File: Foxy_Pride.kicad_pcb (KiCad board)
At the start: 2 copper layers, 89.3 x 67.9 mm, 34 parts, among them U1 TLC555CDR, U2 74HC4017D

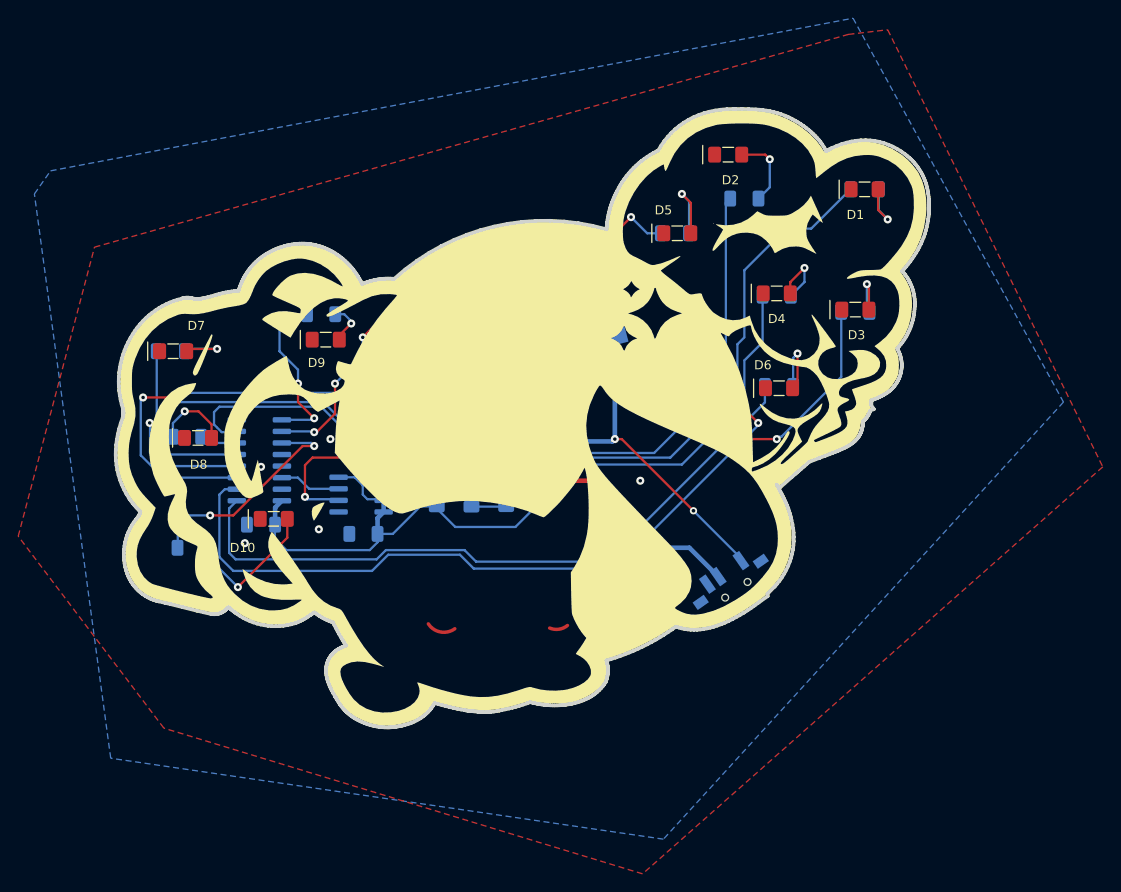
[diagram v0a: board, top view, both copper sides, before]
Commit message: Finalized design and layout on Foxy Pride PCB
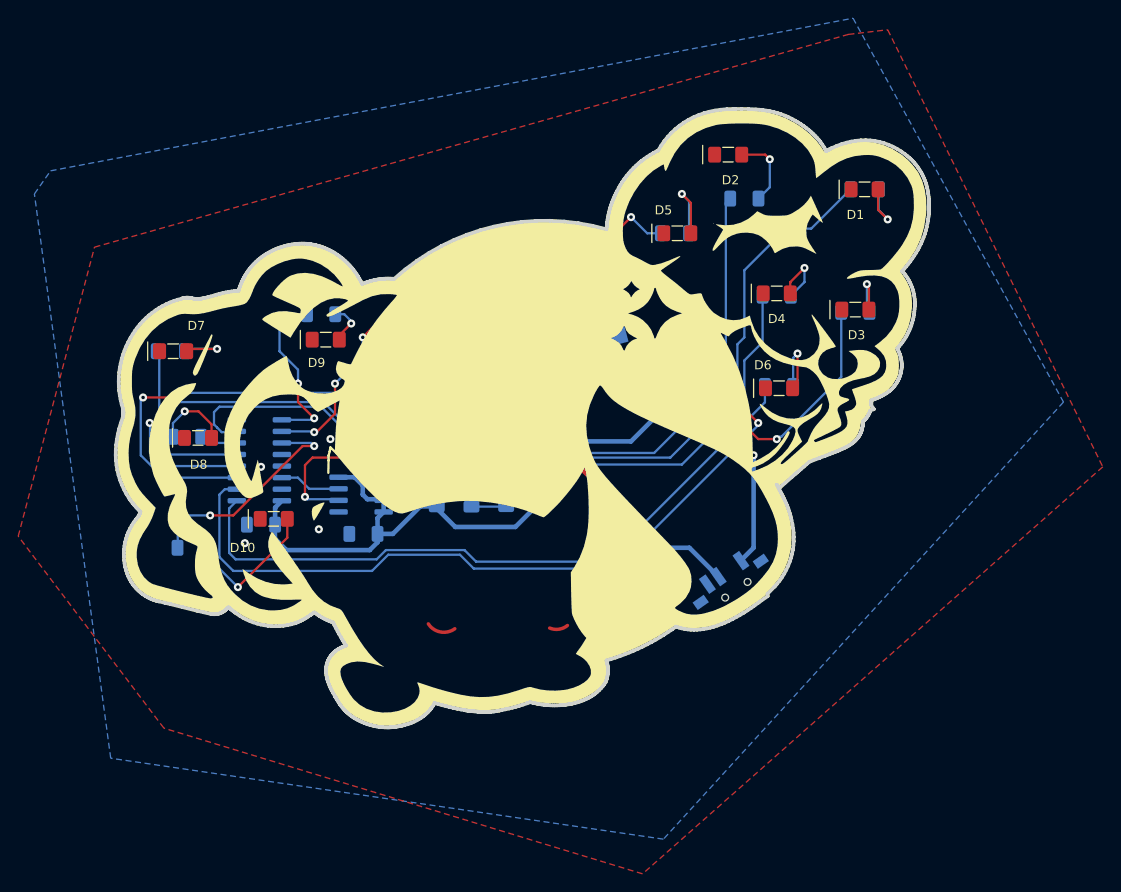
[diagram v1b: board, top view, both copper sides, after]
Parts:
- added G***: LOGO, FoxyPride:Robyn Edit tip of tail 0.73x0.72, F.Cu at (87.4, 74.0)
- added G***: LOGO, FoxyPride:Robyn Edit Ears 1.09x.36, F.Cu at (64.1, 80.1)
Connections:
- S1 pad : (no net) -> GND
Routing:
- net +Vbatt: track 62.6 -> 72.5 mm
- net +3V: track 74.2 -> 77.0 mm
- net GND: vias 11 -> 10
